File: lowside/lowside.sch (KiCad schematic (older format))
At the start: 5 parts, among them J1 Conn_02x39_Odd_Even

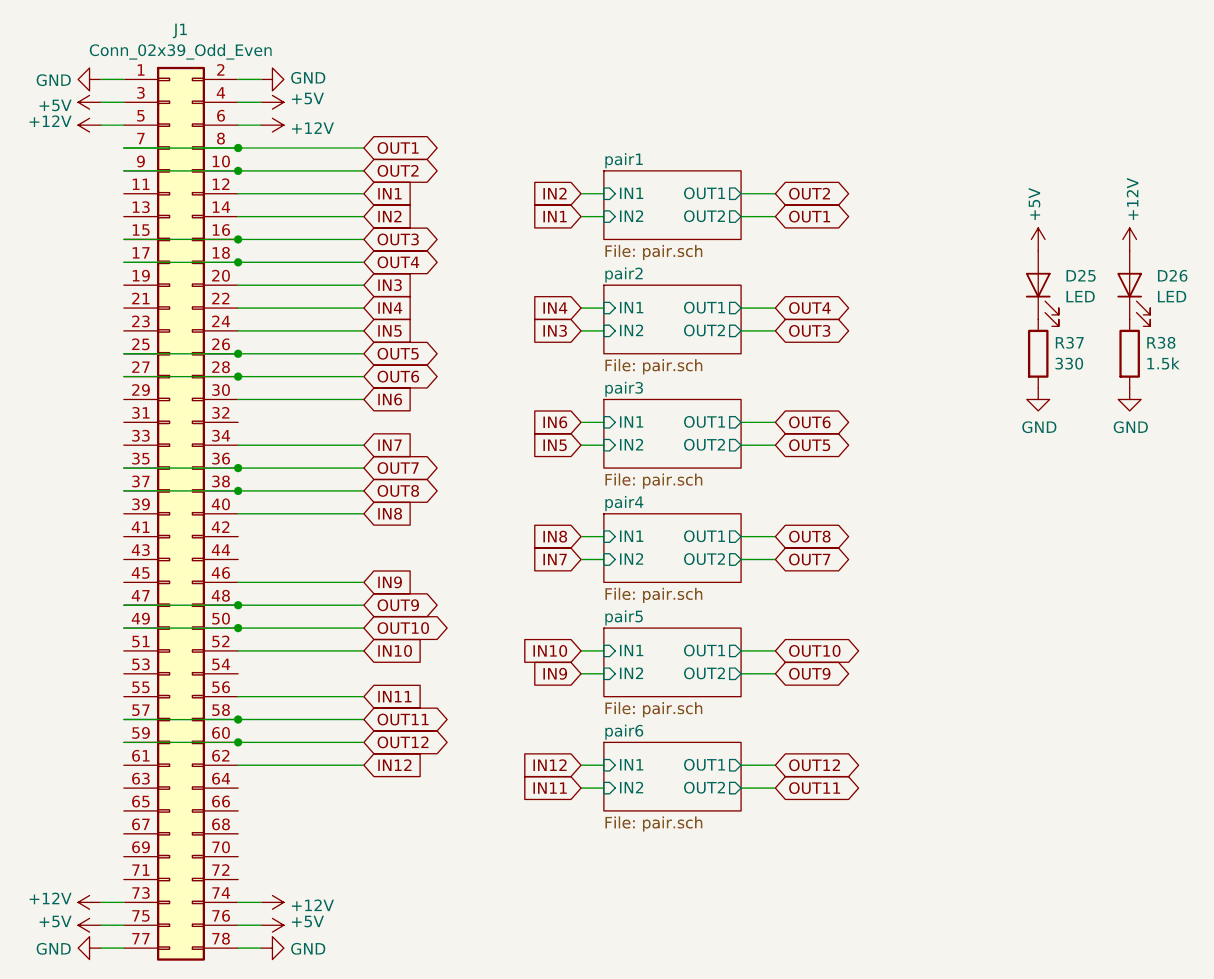
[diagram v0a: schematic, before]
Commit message: add 7th pair
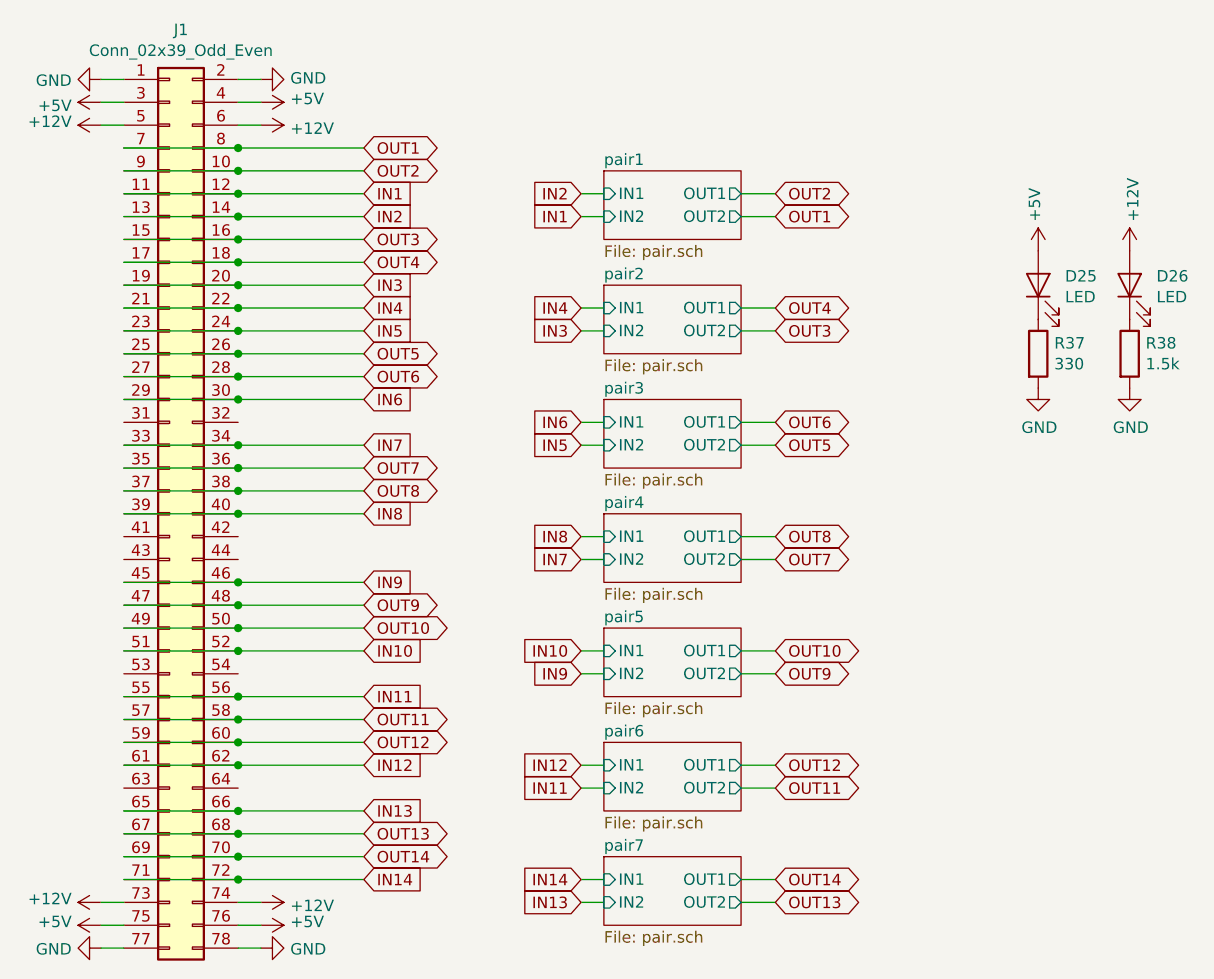
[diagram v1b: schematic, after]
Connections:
- net IN1: now also J1.11 (Pin_11)
- net IN10: now also J1.51 (Pin_51)
- net IN11: now also J1.55 (Pin_55)
- net IN12: now also J1.61 (Pin_61)
- net IN2: now also J1.13 (Pin_13)
- net IN3: now also J1.19 (Pin_19)
- net IN4: now also J1.21 (Pin_21)
- net IN5: now also J1.23 (Pin_23)
- net IN6: now also J1.29 (Pin_29)
- net IN7: now also J1.33 (Pin_33)
- net IN8: now also J1.39 (Pin_39)
- net IN9: now also J1.45 (Pin_45)
- net IN13: now reaches J1.65 (Pin_65)
- net IN13: now also J1.66 (Pin_66)
- net OUT13: now reaches J1.67 (Pin_67)
- net OUT13: now also J1.68 (Pin_68)
- net OUT14: now reaches J1.69 (Pin_69)
- net OUT14: now also J1.70 (Pin_70)
- net IN14: now reaches J1.71 (Pin_71)
- net IN14: now also J1.72 (Pin_72)
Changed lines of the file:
@@
 $Descr A4 11693 8268
 encoding utf-8
-Sheet 1 7
+Sheet 1 8
 Title ""
 Date ""
@@
 	1    0    0    -1
 $EndComp
+$Sheet
+S 4150 5300 600  300
+U 5E2B6330
+F0 "pair7" 50
+F1 "pair.sch" 50
+F2 "IN1" I L 4150 5400 50
+F3 "IN2" I L 4150 5500 50
+F4 "OUT1" O R 4750 5400 50
+F5 "OUT2" O R 4750 5500 50
+$EndSheet
+Text GLabel 4900 5500 2    50   BiDi ~ 0
+OUT13
+Text GLabel 4900 5400 2    50   BiDi ~ 0
+OUT14
+Wire Wire Line
+	4900 5500 4750 5500
+Wire Wire Line
+	4750 5400 4900 5400
+Text GLabel 4050 5500 0    50   Input ~ 0
+IN13
+Wire Wire Line
+	4050 5500 4150 5500
+Wire Wire Line
+	4150 5400 4050 5400
+Text GLabel 4050 5400 0    50   Input ~ 0
+IN14
+Text GLabel 3100 5400 2    50   Input ~ 0
+IN14
+Text GLabel 3100 5100 2    50   Input ~ 0
+IN13
+Text GLabel 3100 5300 2    50   BiDi ~ 0
+OUT14
+Text GLabel 3100 5200 2    50   BiDi ~ 0
+OUT13
+Wire Wire Line
+	3100 5200 2550 5200
+Wire Wire Line
+	3100 5300 2550 5300
+Wire Wire Line
+	2550 5300 2050 5300
+Connection ~ 2550 5300
+Wire Wire Line
+	2050 5200 2550 5200
+Connection ~ 2550 5200
+Wire Wire Line
+	3100 5100 2550 5100
+Wire Wire Line
+	3100 5400 2550 5400
+Wire Wire Line
+	2050 2400 2550 2400
+Connection ~ 2550 2400
+Wire Wire Line
+	2550 2500 2050 2500
+Connection ~ 2550 2500
+Wire Wire Line
+	2050 2800 2550 2800
+Connection ~ 2550 2800
+Wire Wire Line
+	2550 2900 2050 2900
+Connection ~ 2550 2900
+Wire Wire Line
+	2050 3000 2550 3000
+Connection ~ 2550 3000
+Wire Wire Line
+	2050 3300 2550 3300
+Connection ~ 2550 3300
+Wire Wire Line
+	2050 3500 2550 3500
+Connection ~ 2550 3500
+Wire Wire Line
+	2050 3800 2550 3800
+Connection ~ 2550 3800
+Wire Wire Line
+	2050 4100 2550 4100
+Connection ~ 2550 4100
+Wire Wire Line
+	2550 4400 2050 4400
+Connection ~ 2550 4400
+Wire Wire Line
+	2550 4600 2050 4600
+Connection ~ 2550 4600
+Wire Wire Line
+	2550 4900 2050 4900
+Connection ~ 2550 4900
+Wire Wire Line
+	2550 5100 2050 5100
+Connection ~ 2550 5100
+Wire Wire Line
+	2550 5400 2050 5400
+Connection ~ 2550 5400
 $EndSCHEMATC

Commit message: Updated properties in schematic closer to allowing BOM export.
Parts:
- D25, D26: MFG,MFG# (none) -> DIALIGHT,598-8010-107F; Vend1,Vend1# (none) -> DIGI,350-2029-1-ND
- R37: MFG,MFG# (none) -> YAGEO,RC0603FR-07330RL; Vend1,Vend1# (none) -> DIGI,311-330HRCT-ND
- R38: MFG,MFG# (none) -> YAGEO,RC0603JR-071K5L; Vend1,Vend1# (none) -> DIGI,311-1.5KGRCT-ND
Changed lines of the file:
@@
 F 2 "LED_SMD:LED_0603_1608Metric" H 6050 2800 50  0001 C CNN
 F 3 "~" H 6050 2800 50  0001 C CNN
+F 4 "DIALIGHT,598-8010-107F" H 6050 2800 50  0001 C CNN "MFG,MFG#"
+F 5 "DIGI,350-2029-1-ND" H 6050 2800 50  0001 C CNN "Vend1,Vend1#"
 	1    6050 2800
 	0    -1   -1   0
@@
 F 2 "Resistor_SMD:R_0603_1608Metric" V 5980 3100 50  0001 C CNN
 F 3 "~" H 6050 3100 50  0001 C CNN
+F 4 "YAGEO,RC0603FR-07330RL" H 6050 3100 50  0001 C CNN "MFG,MFG#"
+F 5 "DIGI,311-330HRCT-ND" H 6050 3100 50  0001 C CNN "Vend1,Vend1#"
 	1    6050 3100
 	1    0    0    -1
@@
 F 2 "LED_SMD:LED_0603_1608Metric" H 6450 2800 50  0001 C CNN
 F 3 "~" H 6450 2800 50  0001 C CNN
+F 4 "DIALIGHT,598-8010-107F" H 6450 2800 50  0001 C CNN "MFG,MFG#"
+F 5 "DIGI,350-2029-1-ND" H 6450 2800 50  0001 C CNN "Vend1,Vend1#"
 	1    6450 2800
 	0    -1   -1   0
@@
 F 2 "Resistor_SMD:R_0603_1608Metric" V 6380 3100 50  0001 C CNN
 F 3 "~" H 6450 3100 50  0001 C CNN
+F 4 "YAGEO,RC0603JR-071K5L" H 6450 3100 50  0001 C CNN "MFG,MFG#"
+F 5 "DIGI,311-1.5KGRCT-ND" H 6450 3100 50  0001 C CNN "Vend1,Vend1#"
 	1    6450 3100
 	1    0    0    -1

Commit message: getting ready for assembly
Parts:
- D25, D26: LCSC (none) -> C2286
- R37: LCSC (none) -> C416701
- R38: LCSC (none) -> C25867
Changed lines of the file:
@@
 EESchema Schematic File Version 4
-EELAYER 30 0
+LIBS:lowside-cache
+EELAYER 29 0
 EELAYER END
 $Descr A 11000 8500
@@
 F 4 "DIALIGHT,598-8010-107F" H 6050 2800 50  0001 C CNN "MFG,MFG#"
 F 5 "DIGI,350-2029-1-ND" H 6050 2800 50  0001 C CNN "Vend1,Vend1#"
+F 6 "C2286" V 6050 2800 50  0001 C CNN "LCSC"
 	1    6050 2800
 	0    -1   -1   0
@@
 F 4 "YAGEO,RC0603FR-07330RL" H 6050 3100 50  0001 C CNN "MFG,MFG#"
 F 5 "DIGI,311-330HRCT-ND" H 6050 3100 50  0001 C CNN "Vend1,Vend1#"
+F 6 "C416701" H 6050 3100 50  0001 C CNN "LCSC"
 	1    6050 3100
 	1    0    0    -1
@@
 F 4 "DIALIGHT,598-8010-107F" H 6450 2800 50  0001 C CNN "MFG,MFG#"
 F 5 "DIGI,350-2029-1-ND" H 6450 2800 50  0001 C CNN "Vend1,Vend1#"
+F 6 "C2286" V 6450 2800 50  0001 C CNN "LCSC"
 	1    6450 2800
 	0    -1   -1   0
@@
 F 4 "YAGEO,RC0603JR-071K5L" H 6450 3100 50  0001 C CNN "MFG,MFG#"
 F 5 "DIGI,311-1.5KGRCT-ND" H 6450 3100 50  0001 C CNN "Vend1,Vend1#"
+F 6 "C25867" H 6450 3100 50  0001 C CNN "LCSC"
 	1    6450 3100
 	1    0    0    -1
